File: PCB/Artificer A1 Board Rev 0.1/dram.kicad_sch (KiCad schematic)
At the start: 1 part, among them U4 K4F6E3S4HM-MGCJ

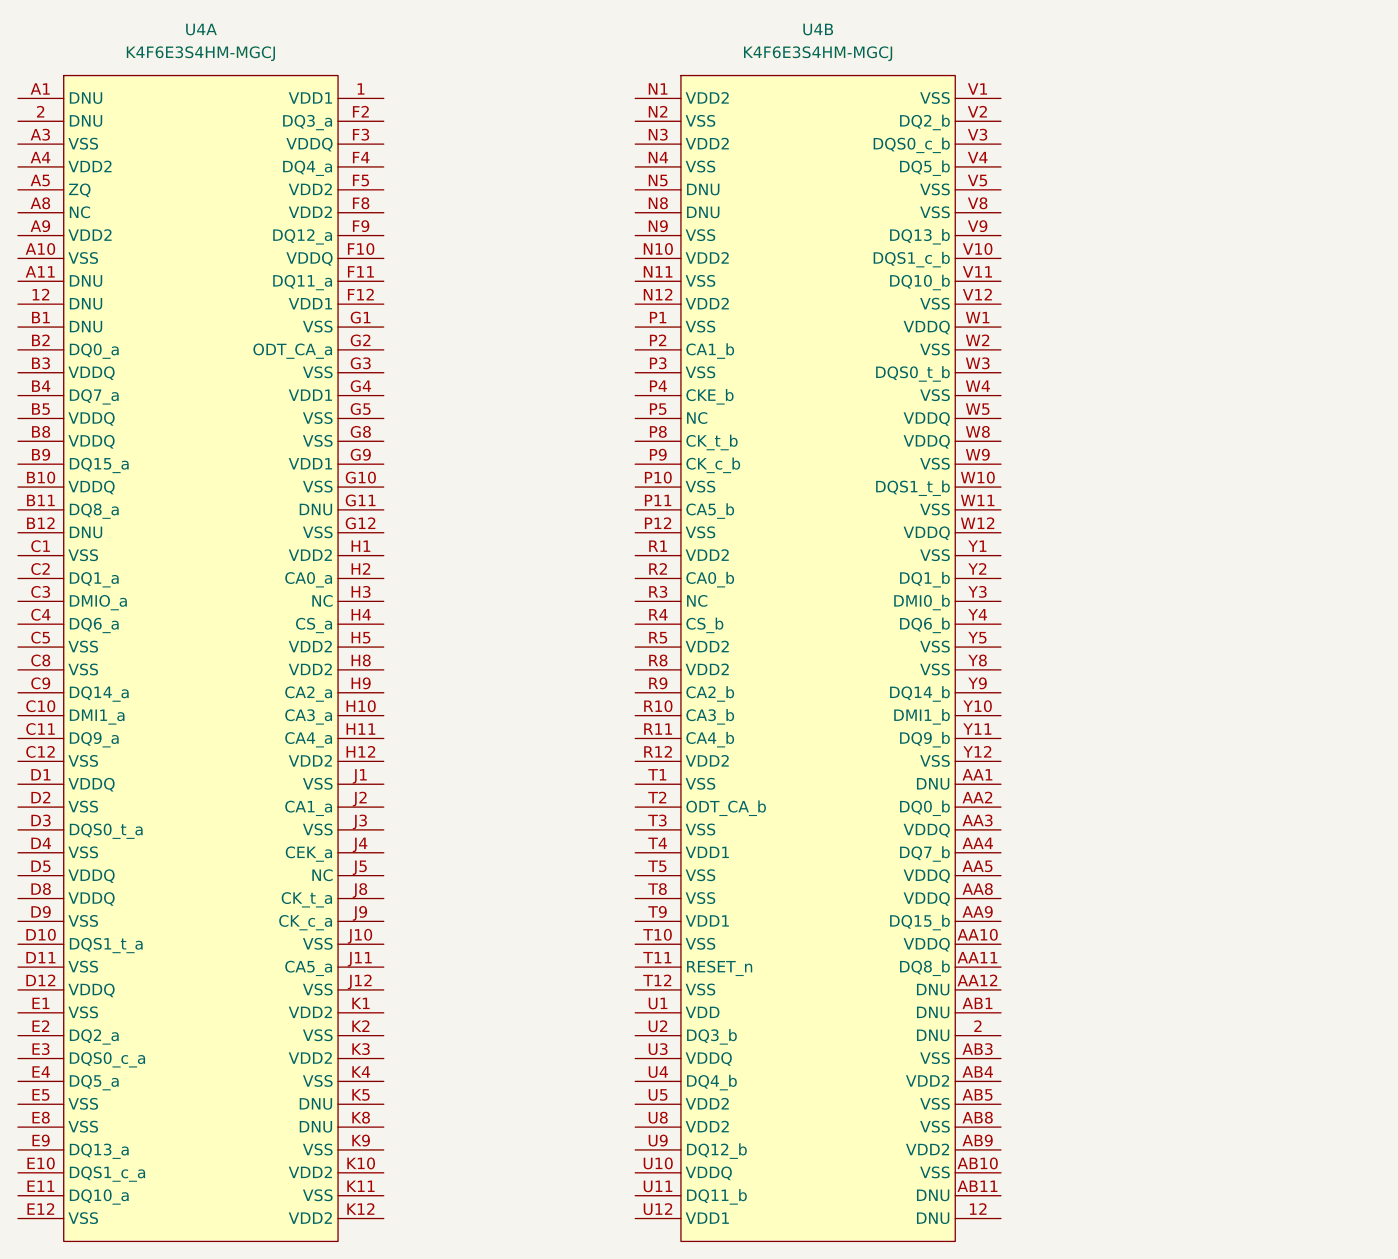
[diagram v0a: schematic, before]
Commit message: added a few accessories
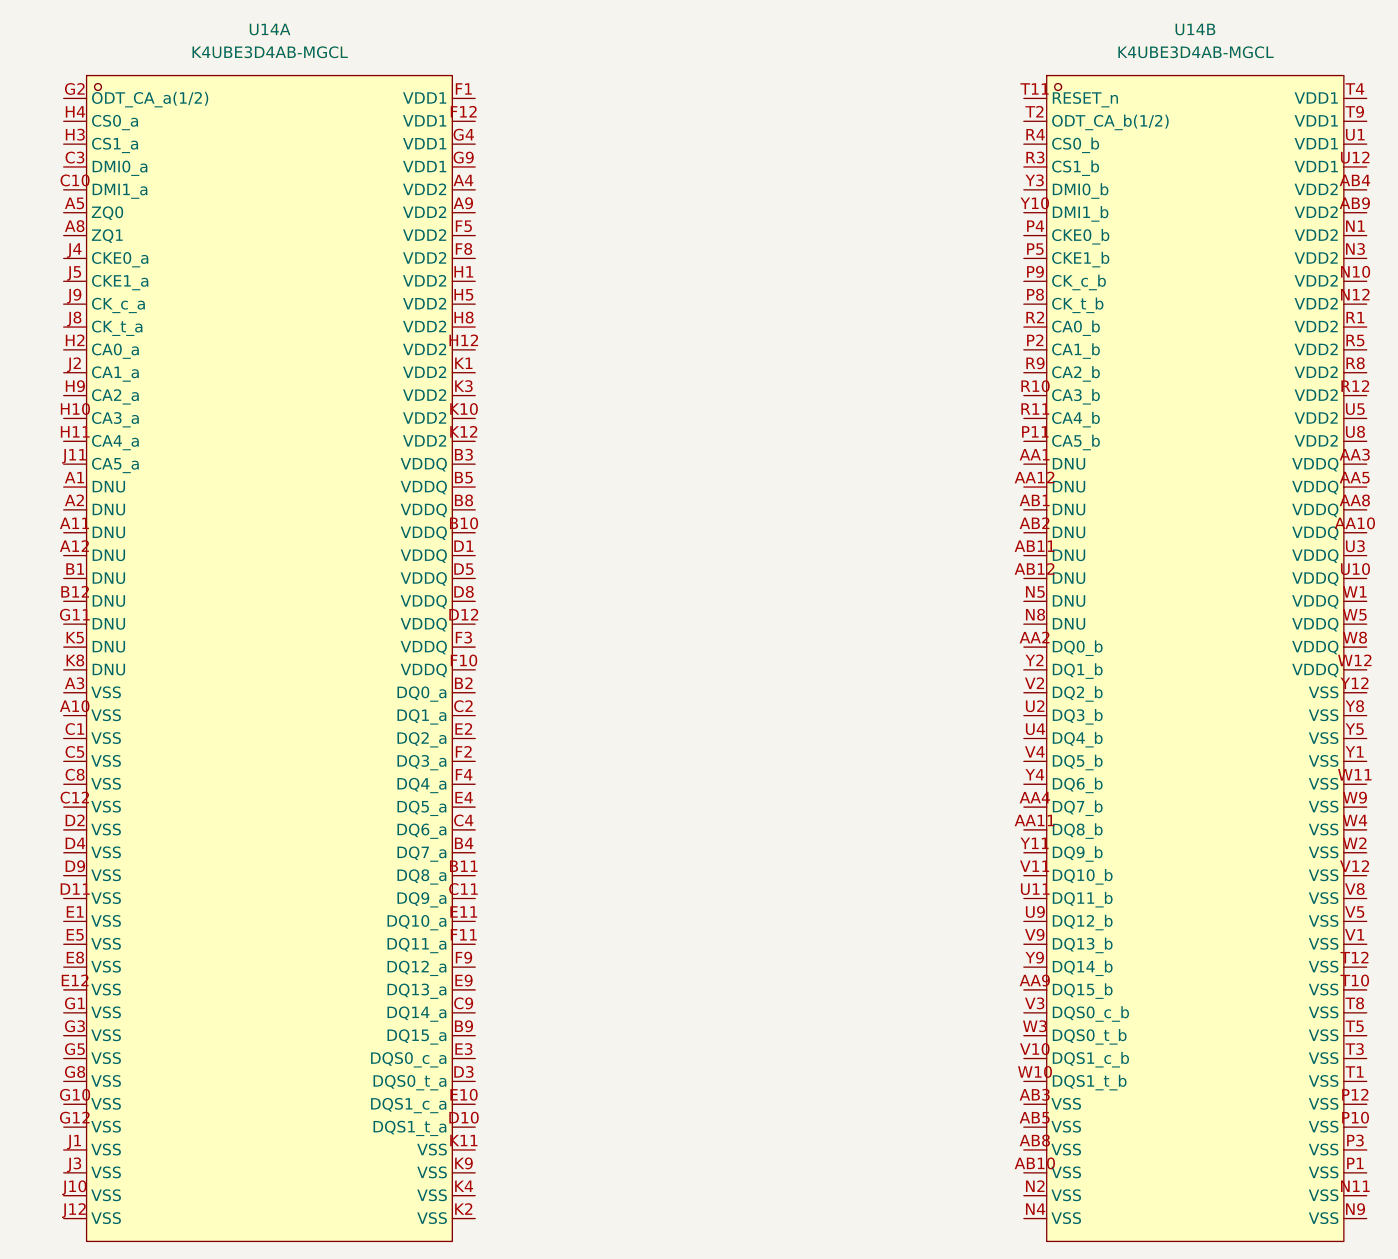
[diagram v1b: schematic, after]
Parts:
- removed U4: K4F6E3S4HM-MGCJ, easyeda:FBGA-200_L15.0-W10.0-BL_K4F6E3S4HM, symbol easyeda:K4F6E3S4HM-MGCJ
- added U14: K4UBE3D4AB-MGCL, easyeda:FBGA-200_L14.5-W10.0_RS1G32LF4D2BDS-53BT, symbol easyeda:K4UBE3D4AB-MGCL
